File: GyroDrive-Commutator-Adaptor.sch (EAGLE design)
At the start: 17 parts, among them IC1 INA2141U, IC2 INA2141U, IC3 INA2141U

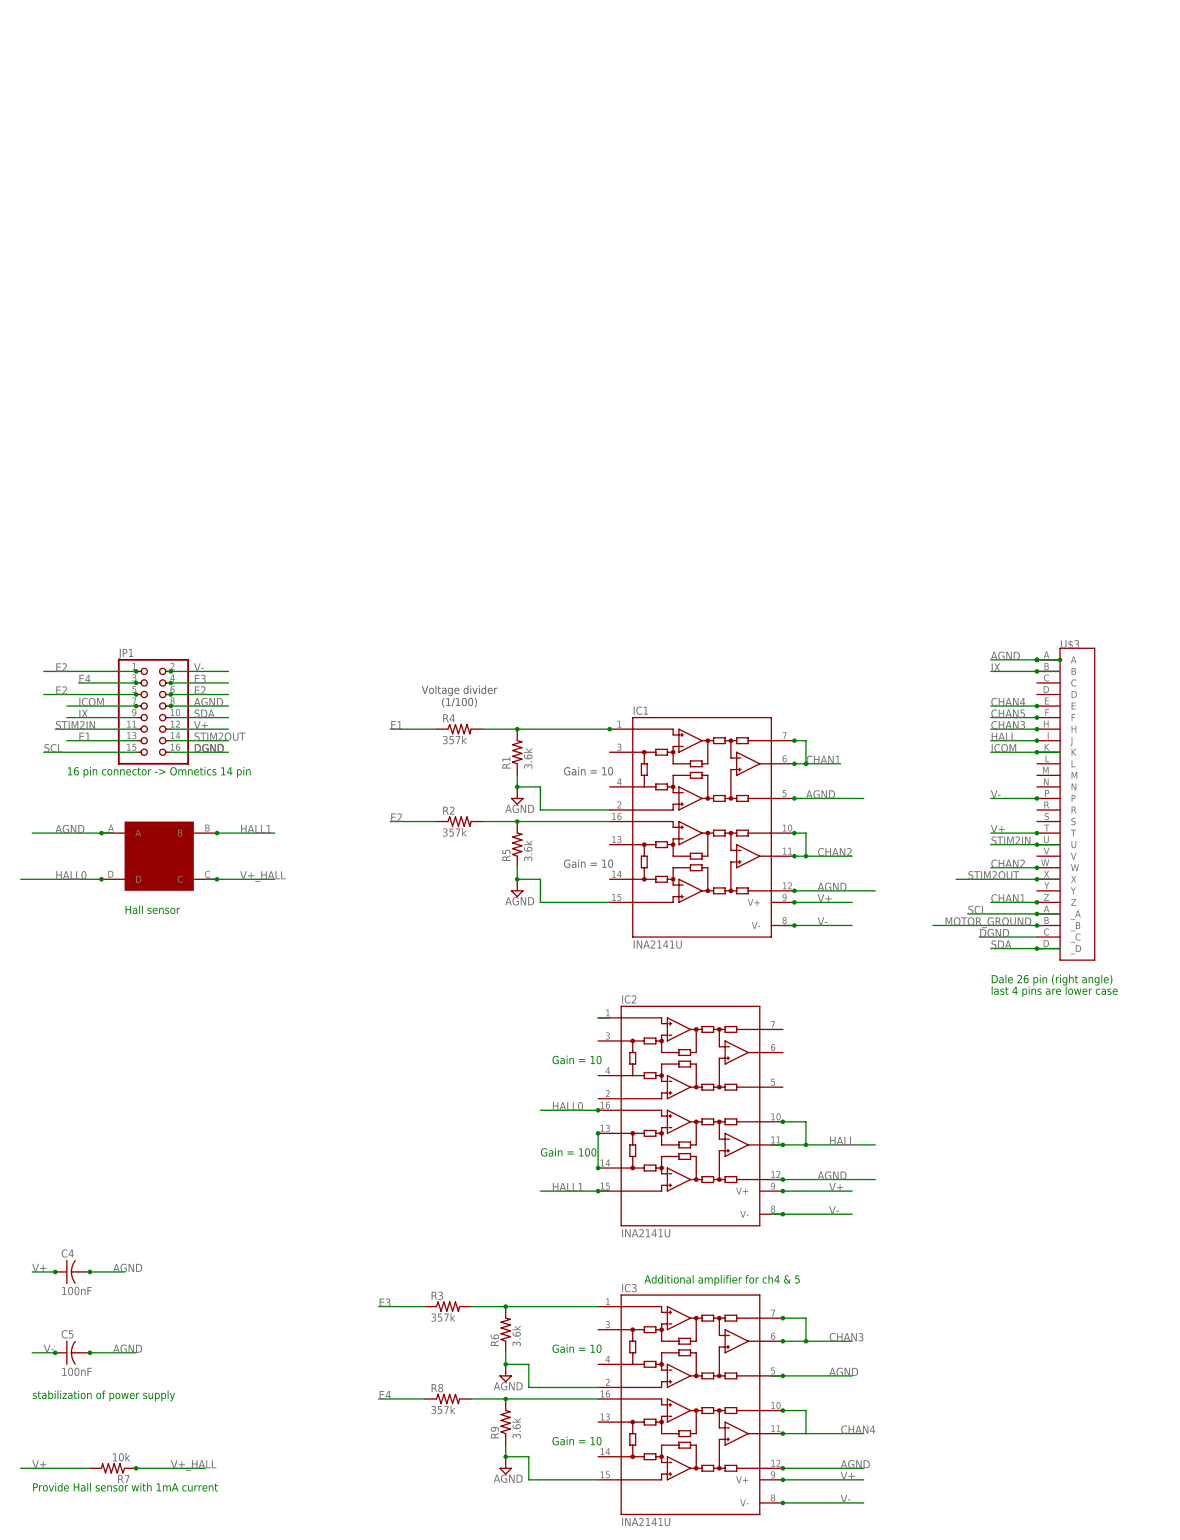
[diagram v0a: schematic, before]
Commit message: Finished routing
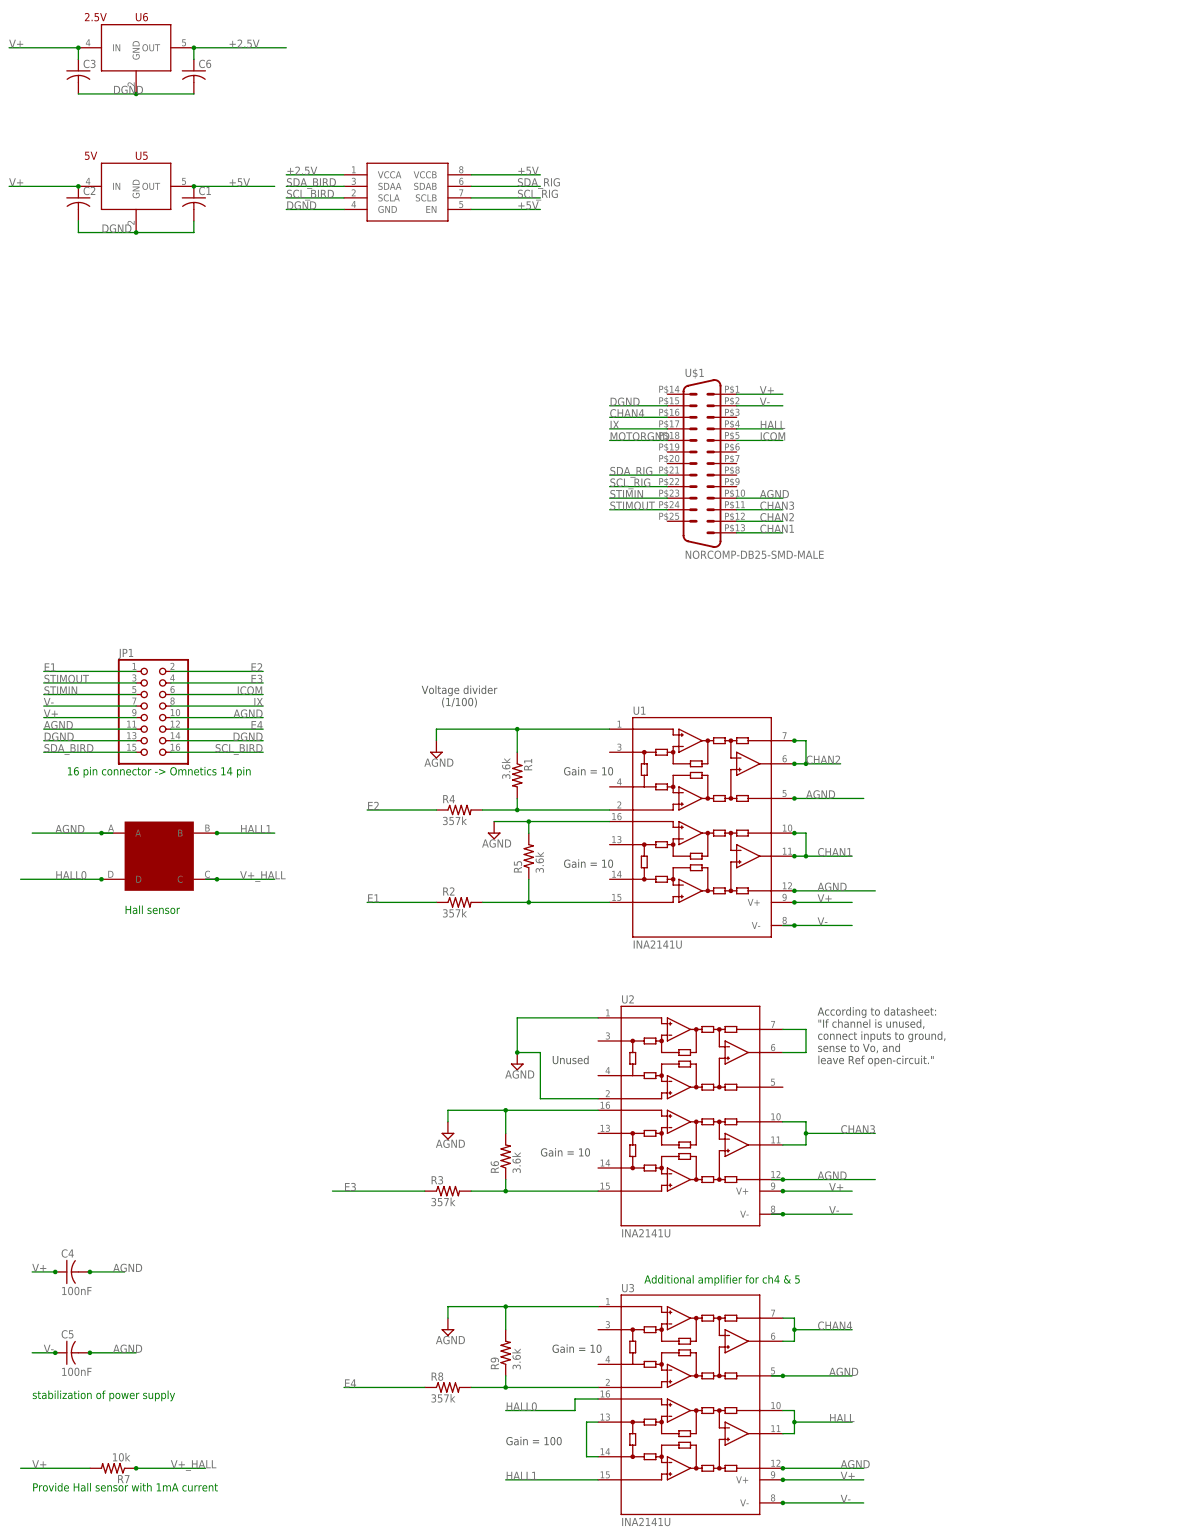
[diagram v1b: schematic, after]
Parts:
- removed U$3: MMD1P22G-26-M101, elm:MMD1P22G-26-M101
- added C1, C2, C3, C6: (no value), resistor:C-USC0402
- added U$1: NORCOMP-DB25-SMD-MALE, michael-stetner:NORCOMP-DB25-SMD-MALE
- added U4: PCA9517, PCA9517:PCA9517
- added U5: 5V, michael-stetner:TPS715-FIXED
- added U6: 2.5V, michael-stetner:TPS715-FIXED
- renumbered IC1 to U1, IC2 to U2, IC3 to U3
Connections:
- removed net CHAN5: U$3.F
- removed net GAIN_HALL: U2.JB, U2.JB@1
- removed net MOTOR_GROUND: U$3._B
- removed net SCL: JP1.15, U$3._A
- removed net SDA: JP1.10, U$3._D
- removed net STIM2IN: JP1.11, U$3.U
- removed net STIM2OUT: JP1.14, U$3.X
- removed net V-_INA: R1.2, R4.2, U1.INA-
- removed net V-_INA1: R2.2, R5.2, U1.INB-
- removed net V-_INA2: R3.2, R6.2, U3.INA-
- removed net V-_INA3: R8.2, R9.2, U3.INB-
- removed net V-_INC: U2.INA-
- new net +2.5V: C6.1, U4.VCCA, U6.OUT
- new net +5V: C1.1, U4.EN, U4.VCCB, U5.OUT
- new net IN1: R2.2, R5.1, U1.INB+
- new net IN2: R1.2, R4.2, U1.INA+
- new net IN3: R3.2, R6.1, U2.INB+
- new net IN4: R8.2, R9.1, U3.INA+
- new net MOTORGND: U$1.18
- new net N$1: U2.SENSEA, U2.VOA
- new net N$3: U3.JB, U3.JB@1
- new net SCL_BIRD: JP1.16, U4.SCLA
- new net SCL_RIG: U$1.22, U4.SCLB
- new net SDA_BIRD: JP1.15, U4.SDAA
- new net SDA_RIG: U$1.21, U4.SDAB
- new net STIMIN: JP1.5, U$1.23
- new net STIMOUT: JP1.3, U$1.24
- net AGND: now also JP1.10, JP1.11, R5.2, R6.2, R9.2, U$1.10, U1.INA-, U1.INB-, U2.INA+, U2.INA-, U2.INB-, U3.INA-; no longer JP1.8, R5.1, R6.1, R9.1, U$3.A, U1.INA+, U1.INB+, U3.INA+, U3.INB+
- net CHAN1: now also U$1.13, U1.SENSEB, U1.VOB; no longer U$3.Z, U1.SENSEA, U1.VOA
- net CHAN2: now also U$1.12, U1.SENSEA, U1.VOA; no longer U$3.W, U1.SENSEB, U1.VOB
- net CHAN3: now also U$1.11, U2.SENSEB, U2.VOB; no longer U$3.H, U3.SENSEA, U3.VOA
- net CHAN4: now also U$1.16, U3.SENSEA, U3.VOA; no longer U$3.E, U3.SENSEB, U3.VOB
- net DGND: now also C1.2, C2.2, C3.2, C6.2, JP1.13, JP1.14, U$1.15, U4.GND, U5.GND, U6.GND; no longer JP1.16, U$3._C
- net E1: now also JP1.1, R2.1; no longer JP1.13, R4.1
- net E2: now also JP1.2, R4.1; no longer JP1.1, JP1.5, JP1.6, R2.1
- net E4: now also JP1.12; no longer JP1.3
- net HALL: now also U$1.4, U3.SENSEB, U3.VOB; no longer U$3.J, U2.SENSEB, U2.VOB
- net HALL0: now also U3.INB-; no longer U2.INB-
- net HALL1: now also U3.INB+; no longer U2.INB+
- net ICOM: now also JP1.6, U$1.5; no longer JP1.7, U$3.K
- net IX: now also JP1.8, U$1.17; no longer JP1.9, U$3.B
- net V+: now also C2.1, C3.1, JP1.9, U$1.1, U5.IN, U6.IN; no longer JP1.12, U$3.T
- net V-: now also JP1.7, U$1.2; no longer JP1.2, U$3.P
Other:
- note added: "According to datasheet: "If channel is unused, connect inputs to ground, sense to Vo, and leave Ref open-circuit.""
- note added: "Unused"
- note removed: "Dale 26 pin (right angle)"
- note removed: "last 4 pins are lower case"
- moved on the sheet: R1, R2, R3, R4, R5, R6, R8, R9
